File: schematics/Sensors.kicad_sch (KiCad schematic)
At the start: 4 parts, among them U4 HDC1080

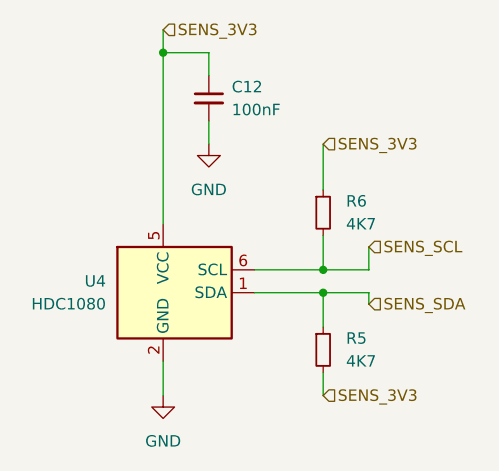
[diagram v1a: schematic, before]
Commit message: connectors
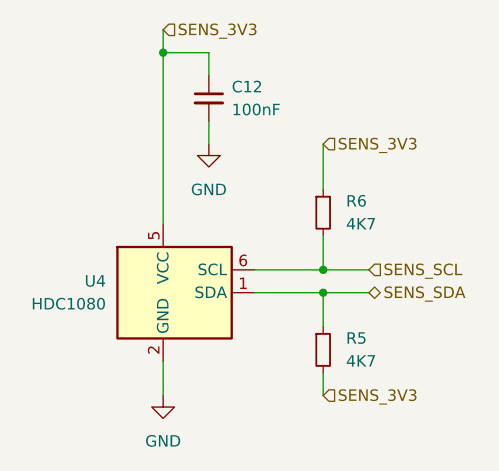
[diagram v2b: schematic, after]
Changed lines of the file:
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@@
-	(wire
-		(pts
-			(xy 172.72 95.25) (xy 172.72 96.52)
-		)
-		(stroke
-			(width 0)
-			(type default)
-		)
-	)
 	(wire
 		(pts
@@
 		(pts
 			(xy 167.64 92.71) (xy 172.72 92.71)
-		)
-		(stroke
-			(width 0)
-			(type default)
-		)
-	)
-	(wire
-		(pts
-			(xy 172.72 92.71) (xy 172.72 90.17)
 		)
 		(stroke
@@
 	)
 	(hierarchical_label "SENS_SDA"
-		(shape input)
-		(at 172.72 96.52 0)
+		(shape bidirectional)
+		(at 172.72 95.25 0)
 		(fields_autoplaced yes)
 		(effects
@@
 	(hierarchical_label "SENS_SCL"
 		(shape input)
-		(at 172.72 90.17 0)
+		(at 172.72 92.71 0)
 		(fields_autoplaced yes)
 		(effects
